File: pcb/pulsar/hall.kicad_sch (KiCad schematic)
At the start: 244 parts, among them U1 DRV5055A2QDBZR, U10 DRV5055A2QDBZR, U11 DRV5055A2QDBZR, U12 DRV5055A2QDBZR, U13 DRV5055A2QDBZR, U14 DRV5055A2QDBZR, U15 DRV5055A2QDBZR, U16 DRV5055A2QDBZR, U17 DRV5055A2QDBZR, U18 DRV5055A2QDBZR, U19 DRV5055A2QDBZR, U2 DRV5055A2QDBZR, U20 DRV5055A2QDBZR, U21 DRV5055A2QDBZR, U22 DRV5055A2QDBZR, U23 DRV5055A2QDBZR, U24 DRV5055A2QDBZR, U25 DRV5055A2QDBZR, U26 DRV5055A2QDBZR, U27 DRV5055A2QDBZR, U28 DRV5055A2QDBZR, U29 DRV5055A2QDBZR, U3 DRV5055A2QDBZR, U30 DRV5055A2QDBZR, U31 DRV5055A2QDBZR, U32 DRV5055A2QDBZR, U33 DRV5055A2QDBZR, U34 DRV5055A2QDBZR, U35 DRV5055A2QDBZR, U36 DRV5055A2QDBZR, U37 DRV5055A2QDBZR, U38 DRV5055A2QDBZR, U39 DRV5055A2QDBZR, U4 DRV5055A2QDBZR, U40 DRV5055A2QDBZR, U41 DRV5055A2QDBZR, U42 DRV5055A2QDBZR, U43 DRV5055A2QDBZR, U44 DRV5055A2QDBZR, U45 DRV5055A2QDBZR, U46 DRV5055A2QDBZR, U47 DRV5055A2QDBZR, U48 DRV5055A2QDBZR, U49 DRV5055A2QDBZR, U5 DRV5055A2QDBZR, U50 DRV5055A2QDBZR, U51 DRV5055A2QDBZR, U52 DRV5055A2QDBZR, U53 DRV5055A2QDBZR, U54 DRV5055A2QDBZR, U55 DRV5055A2QDBZR, U56 DRV5055A2QDBZR, U57 DRV5055A2QDBZR, U58 DRV5055A2QDBZR, U59 DRV5055A2QDBZR, U6 DRV5055A2QDBZR, U60 DRV5055A2QDBZR, U61 DRV5055A2QDBZR, U7 DRV5055A2QDBZR, U8 DRV5055A2QDBZR, U9 DRV5055A2QDBZR

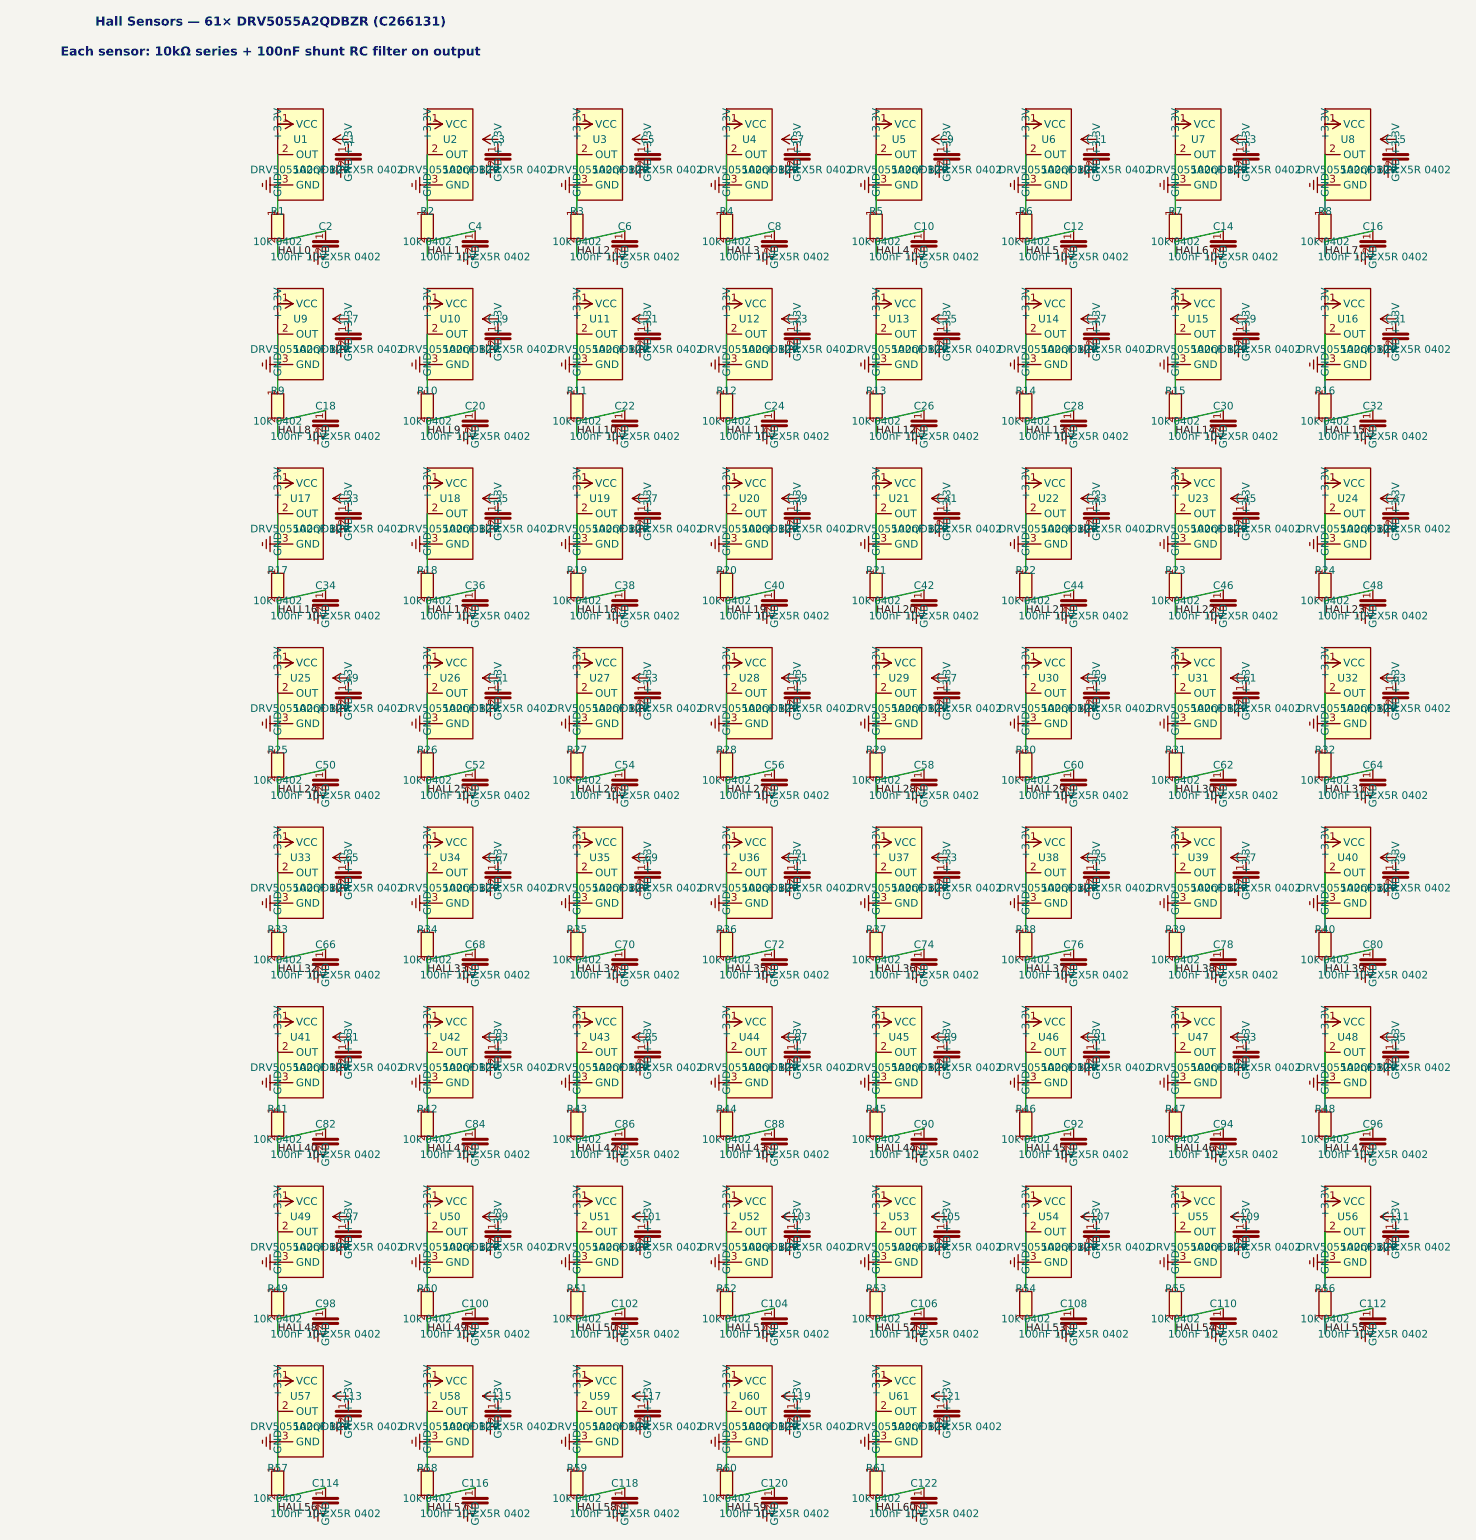
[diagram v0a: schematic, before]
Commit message: feat: let everything to route
Signed-off-by: Axel Ibarrondo <135344010+Axel84727@users.noreply.github.com>
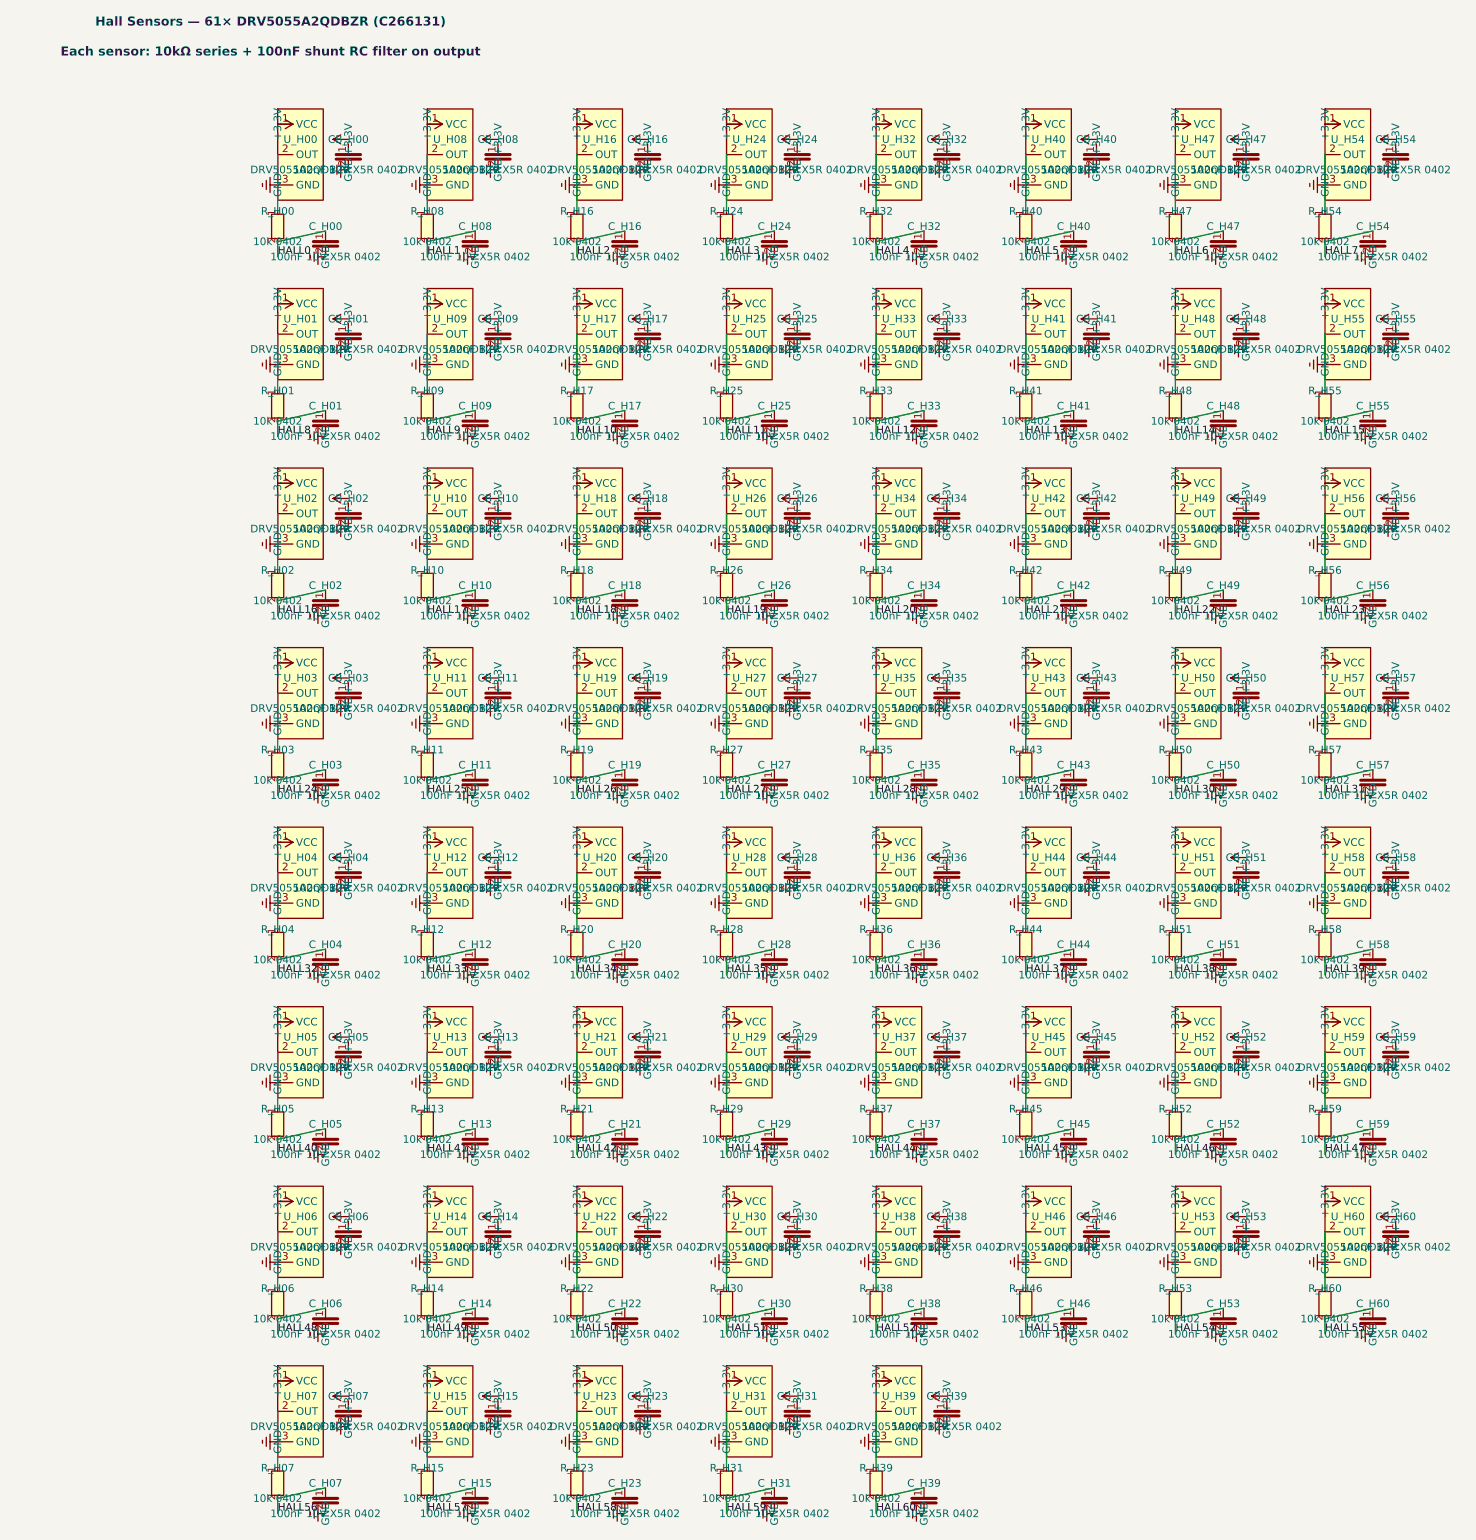
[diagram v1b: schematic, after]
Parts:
- renumbered C1 to CB_H00, C17 to CB_H01, C33 to CB_H02, C49 to CB_H03, C65 to CB_H04, C81 to CB_H05, C97 to CB_H06, C113 to CB_H07, C3 to CB_H08, C19 to CB_H09, C35 to CB_H10, C51 to CB_H11, C67 to CB_H12, C83 to CB_H13, C99 to CB_H14, C115 to CB_H15, C5 to CB_H16, C21 to CB_H17, C37 to CB_H18, C53 to CB_H19, C69 to CB_H20, C85 to CB_H21, C101 to CB_H22, C117 to CB_H23, C7 to CB_H24, C23 to CB_H25, C39 to CB_H26, C55 to CB_H27, C71 to CB_H28, C87 to CB_H29, C103 to CB_H30, C119 to CB_H31, C9 to CB_H32, C25 to CB_H33, C41 to CB_H34, C57 to CB_H35, C73 to CB_H36, C89 to CB_H37, C105 to CB_H38, C121 to CB_H39, C11 to CB_H40, C27 to CB_H41, C43 to CB_H42, C59 to CB_H43, C75 to CB_H44, C91 to CB_H45, C107 to CB_H46, C13 to CB_H47, C29 to CB_H48, C45 to CB_H49, C61 to CB_H50, C77 to CB_H51, C93 to CB_H52, C109 to CB_H53, C15 to CB_H54, C31 to CB_H55, C47 to CB_H56, C63 to CB_H57, C79 to CB_H58, C95 to CB_H59, C111 to CB_H60, C2 to C_H00, C18 to C_H01, C34 to C_H02, C50 to C_H03, C66 to C_H04, C82 to C_H05, C98 to C_H06, C114 to C_H07, C4 to C_H08, C20 to C_H09, C36 to C_H10, C52 to C_H11, C68 to C_H12, C84 to C_H13, C100 to C_H14, C116 to C_H15, C6 to C_H16, C22 to C_H17, C38 to C_H18, C54 to C_H19, C70 to C_H20, C86 to C_H21, C102 to C_H22, C118 to C_H23, C8 to C_H24, C24 to C_H25, C40 to C_H26, C56 to C_H27, C72 to C_H28, C88 to C_H29, C104 to C_H30, C120 to C_H31, C10 to C_H32, C26 to C_H33, C42 to C_H34, C58 to C_H35, C74 to C_H36, C90 to C_H37, C106 to C_H38, C122 to C_H39, C12 to C_H40, C28 to C_H41, C44 to C_H42, C60 to C_H43, C76 to C_H44, C92 to C_H45, C108 to C_H46, C14 to C_H47, C30 to C_H48, C46 to C_H49, C62 to C_H50, C78 to C_H51, C94 to C_H52, C110 to C_H53, C16 to C_H54, C32 to C_H55, C48 to C_H56, C64 to C_H57, C80 to C_H58, C96 to C_H59, C112 to C_H60, R1 to R_H00, R9 to R_H01, R17 to R_H02, R25 to R_H03, R33 to R_H04, R41 to R_H05, R49 to R_H06, R57 to R_H07, R2 to R_H08, R10 to R_H09, R18 to R_H10, R26 to R_H11, R34 to R_H12, R42 to R_H13, R50 to R_H14, R58 to R_H15, R3 to R_H16, R11 to R_H17, R19 to R_H18, R27 to R_H19, R35 to R_H20, R43 to R_H21, R51 to R_H22, R59 to R_H23, R4 to R_H24, R12 to R_H25, R20 to R_H26, R28 to R_H27, R36 to R_H28, R44 to R_H29, R52 to R_H30, R60 to R_H31, R5 to R_H32, R13 to R_H33, R21 to R_H34, R29 to R_H35, R37 to R_H36, R45 to R_H37, R53 to R_H38, R61 to R_H39, R6 to R_H40, R14 to R_H41, R22 to R_H42, R30 to R_H43, R38 to R_H44, R46 to R_H45, R54 to R_H46, R7 to R_H47, R15 to R_H48, R23 to R_H49, R31 to R_H50, R39 to R_H51, R47 to R_H52, R55 to R_H53, R8 to R_H54, R16 to R_H55, R24 to R_H56, R32 to R_H57, R40 to R_H58, R48 to R_H59, R56 to R_H60, U1 to U_H00, U9 to U_H01, U17 to U_H02, U25 to U_H03, U33 to U_H04, U41 to U_H05, U49 to U_H06, U57 to U_H07, U2 to U_H08, U10 to U_H09, U18 to U_H10, U26 to U_H11, U34 to U_H12, U42 to U_H13, U50 to U_H14, U58 to U_H15, U3 to U_H16, U11 to U_H17, U19 to U_H18, U27 to U_H19, U35 to U_H20, U43 to U_H21, U51 to U_H22, U59 to U_H23, U4 to U_H24, U12 to U_H25, U20 to U_H26, U28 to U_H27, U36 to U_H28, U44 to U_H29, U52 to U_H30, U60 to U_H31, U5 to U_H32, U13 to U_H33, U21 to U_H34, U29 to U_H35, U37 to U_H36, U45 to U_H37, U53 to U_H38, U61 to U_H39, U6 to U_H40, U14 to U_H41, U22 to U_H42, U30 to U_H43, U38 to U_H44, U46 to U_H45, U54 to U_H46, U7 to U_H47, U15 to U_H48, U23 to U_H49, U31 to U_H50, U39 to U_H51, U47 to U_H52, U55 to U_H53, U8 to U_H54, U16 to U_H55, U24 to U_H56, U32 to U_H57, U40 to U_H58, U48 to U_H59, U56 to U_H60
